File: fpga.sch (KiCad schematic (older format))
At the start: 18 parts, among them U5 ICE40UP5K-SG48ITR, U6 LY68L6400

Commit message: Change pinout of expansion header close to board edge to be fully ground instead of gnd + 3.3v (& update component references)
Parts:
- C15, C16, C17, C18, C19, C20, C21, C22: symbol Device:C_Small -> mch2021-rescue:C_Small-Device
- R31, R32, R33, R34, R35, R36: symbol Device:R_Small -> mch2021-rescue:R_Small-Device
- RN4, RN5: symbol Device:R_Pack04 -> mch2021-rescue:R_Pack04-Device
- U5: symbol FPGA_Lattice:ICE40UP5K-SG48ITR -> mch2021-rescue:ICE40UP5K-SG48ITR-FPGA_Lattice
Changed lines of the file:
@@
 $EndDescr
 $Comp
-L FPGA_Lattice:ICE40UP5K-SG48ITR U5
+L mch2021-rescue:ICE40UP5K-SG48ITR-FPGA_Lattice U5
 U 1 1 5F52B856
 P 1850 6100
@@
 $EndComp
 $Comp
-L FPGA_Lattice:ICE40UP5K-SG48ITR U5
+L mch2021-rescue:ICE40UP5K-SG48ITR-FPGA_Lattice U5
 U 2 1 5F52DB74
 P 3500 6100
@@
 $EndComp
 $Comp
-L FPGA_Lattice:ICE40UP5K-SG48ITR U5
+L mch2021-rescue:ICE40UP5K-SG48ITR-FPGA_Lattice U5
 U 3 1 5F52F020
 P 9000 3900
@@
 $EndComp
 $Comp
-L FPGA_Lattice:ICE40UP5K-SG48ITR U5
+L mch2021-rescue:ICE40UP5K-SG48ITR-FPGA_Lattice U5
 U 4 1 5F5301DA
 P 2650 1200
@@
 $EndComp
 $Comp
-L Device:R_Small R33
+L mch2021-rescue:R_Small-Device R33
 U 1 1 5F537E5C
 P 1700 1350
@@
 $EndComp
 $Comp
-L Device:C_Small C16
+L mch2021-rescue:C_Small-Device C16
 U 1 1 5F54E79A
 P 1300 1700
@@
 $EndComp
 $Comp
-L Device:C_Small C17
+L mch2021-rescue:C_Small-Device C17
 U 1 1 5F54FA10
 P 1700 1700
@@
 $EndComp
 $Comp
-L Device:C_Small C18
+L mch2021-rescue:C_Small-Device C18
 U 1 1 5F551B90
 P 2100 1700
@@
 $EndComp
 $Comp
-L power:GND #PWR084
+L mch2021-rescue:GND-power #PWR084
 U 1 1 5F553535
 P 2100 1800
@@
 $EndComp
 $Comp
-L power:GND #PWR080
+L mch2021-rescue:GND-power #PWR080
 U 1 1 5F553952
 P 1700 1800
@@
 $EndComp
 $Comp
-L power:GND #PWR078
+L mch2021-rescue:GND-power #PWR078
 U 1 1 5F553E39
 P 1300 1800
@@
 Connection ~ 1300 1200
 $Comp
-L power:+1V2 #PWR075
+L mch2021-rescue:+1V2-power #PWR075
 U 1 1 5F564804
 P 900 1000
@@
 $EndComp
 $Comp
-L power:GND #PWR088
+L mch2021-rescue:GND-power #PWR088
 U 1 1 5F565850
 P 3150 1800
@@
 	3150 1200 3050 1200
 $Comp
-L power:+3.3V #PWR091
+L mch2021-rescue:+3.3V-power #PWR091
 U 1 1 5F57B8C0
 P 3500 5000
@@
 FPGA_CDONE
 $Comp
-L power:GND #PWR077
+L mch2021-rescue:GND-power #PWR077
 U 1 1 5F58383F
 P 1100 3150
@@
 $EndComp
 $Comp
-L Device:R_Small R31
+L mch2021-rescue:R_Small-Device R31
 U 1 1 5F59314F
 P 1100 3050
@@
 FPGA_RESET
 $Comp
-L Device:R_Small R32
+L mch2021-rescue:R_Small-Device R32
 U 1 1 5F5BBEB5
 P 1400 2700
@@
 FPGA_CDONE
 $Comp
-L power:+3.3V #PWR079
+L mch2021-rescue:+3.3V-power #PWR079
 U 1 1 5F5BD259
 P 1400 2600
@@
 LCD_FMARK
 $Comp
-L power:+3.3V #PWR082
+L mch2021-rescue:+3.3V-power #PWR082
 U 1 1 60CF7467
 P 1850 5000
@@
 RGB0
 $Comp
-L power:+3.3V #PWR094
+L mch2021-rescue:+3.3V-power #PWR094
 U 1 1 5F32B7AB
 P 9000 3200
@@
 	10500 1750 10500 1800
 $Comp
-L power:GND #PWR099
+L mch2021-rescue:GND-power #PWR099
 U 1 1 5F3AAB21
 P 10500 1800
@@
 $EndComp
 $Comp
-L Device:R_Small R36
+L mch2021-rescue:R_Small-Device R36
 U 1 1 5F436AA9
 P 9450 1050
@@
 	9450 1250 9450 1150
 $Comp
-L power:+3.3V #PWR095
+L mch2021-rescue:+3.3V-power #PWR095
 U 1 1 5F439DDC
 P 9450 950
@@
 $EndComp
 $Comp
-L power:+3.3V #PWR098
+L mch2021-rescue:+3.3V-power #PWR098
 U 1 1 5F43A076
 P 10500 950
@@
 	9550 1750 9350 1750
 $Comp
-L Device:C_Small C21
+L mch2021-rescue:C_Small-Device C21
 U 1 1 5F472EE7
 P 4700 5100
@@
 $EndComp
 $Comp
-L power:GND #PWR093
+L mch2021-rescue:GND-power #PWR093
 U 1 1 5F473D9D
 P 4700 5200
@@
 $EndComp
 $Comp
-L power:+3.3V #PWR092
+L mch2021-rescue:+3.3V-power #PWR092
 U 1 1 5F473F7E
 P 4700 5000
@@
 $EndComp
 $Comp
-L Device:C_Small C22
+L mch2021-rescue:C_Small-Device C22
 U 1 1 5F47D064
 P 9550 3300
@@
 $EndComp
 $Comp
-L power:GND #PWR097
+L mch2021-rescue:GND-power #PWR097
 U 1 1 5F47D06A
 P 9550 3400
@@
 $EndComp
 $Comp
-L power:+3.3V #PWR096
+L mch2021-rescue:+3.3V-power #PWR096
 U 1 1 5F47D070
 P 9550 3200
@@
 $EndComp
 $Comp
-L Device:C_Small C20
+L mch2021-rescue:C_Small-Device C20
 U 1 1 5F47E26A
 P 3450 1700
@@
 $EndComp
 $Comp
-L power:GND #PWR090
+L mch2021-rescue:GND-power #PWR090
 U 1 1 5F47E270
 P 3450 1800
@@
 $EndComp
 $Comp
-L power:+3.3V #PWR089
+L mch2021-rescue:+3.3V-power #PWR089
 U 1 1 5F47E276
 P 3450 1600
@@
 $EndComp
 $Comp
-L Device:C_Small C19
+L mch2021-rescue:C_Small-Device C19
 U 1 1 5F489EE6
 P 2300 5100
@@
 $EndComp
 $Comp
-L power:GND #PWR087
+L mch2021-rescue:GND-power #PWR087
 U 1 1 5F489EEC
 P 2300 5200
@@
 $EndComp
 $Comp
-L power:+3.3V #PWR086
+L mch2021-rescue:+3.3V-power #PWR086
 U 1 1 5F489EF2
 P 2300 5000
@@
 $EndComp
 $Comp
-L Device:C_Small C15
+L mch2021-rescue:C_Small-Device C15
 U 1 1 5F48A8F4
 P 900 1700
@@
 $EndComp
 $Comp
-L power:GND #PWR076
+L mch2021-rescue:GND-power #PWR076
 U 1 1 5F48A8FA
 P 900 1800
@@
 PMOD_7
 $Comp
-L Device:R_Pack04 RN5
+L mch2021-rescue:R_Pack04-Device RN5
 U 1 1 5FD85945
 P 7300 4300
@@
 IRQ
 $Comp
-L Device:R_Small R34
+L mch2021-rescue:R_Small-Device R34
 U 1 1 5F54C08B
 P 1750 2700
@@
 $EndComp
 $Comp
-L power:+3.3V #PWR081
+L mch2021-rescue:+3.3V-power #PWR081
 U 1 1 5F54C091
 P 1750 2600
@@
 RGB1
 $Comp
-L Device:R_Small R35
+L mch2021-rescue:R_Small-Device R35
 U 1 1 5F503F4E
 P 2050 2700
@@
 SPI_CS
 $Comp
-L power:+3.3V #PWR083
+L mch2021-rescue:+3.3V-power #PWR083
 U 1 1 5F89A681
 P 2050 2600
@@
 $EndComp
 $Comp
-L power:+3.3V #PWR085
+L mch2021-rescue:+3.3V-power #PWR085
 U 1 1 5F8E28AC
 P 2250 1100
@@
 I2S_LR
 $Comp
-L Device:R_Pack04 RN4
+L mch2021-rescue:R_Pack04-Device RN4
 U 1 1 5FD84D43
 P 7300 3900

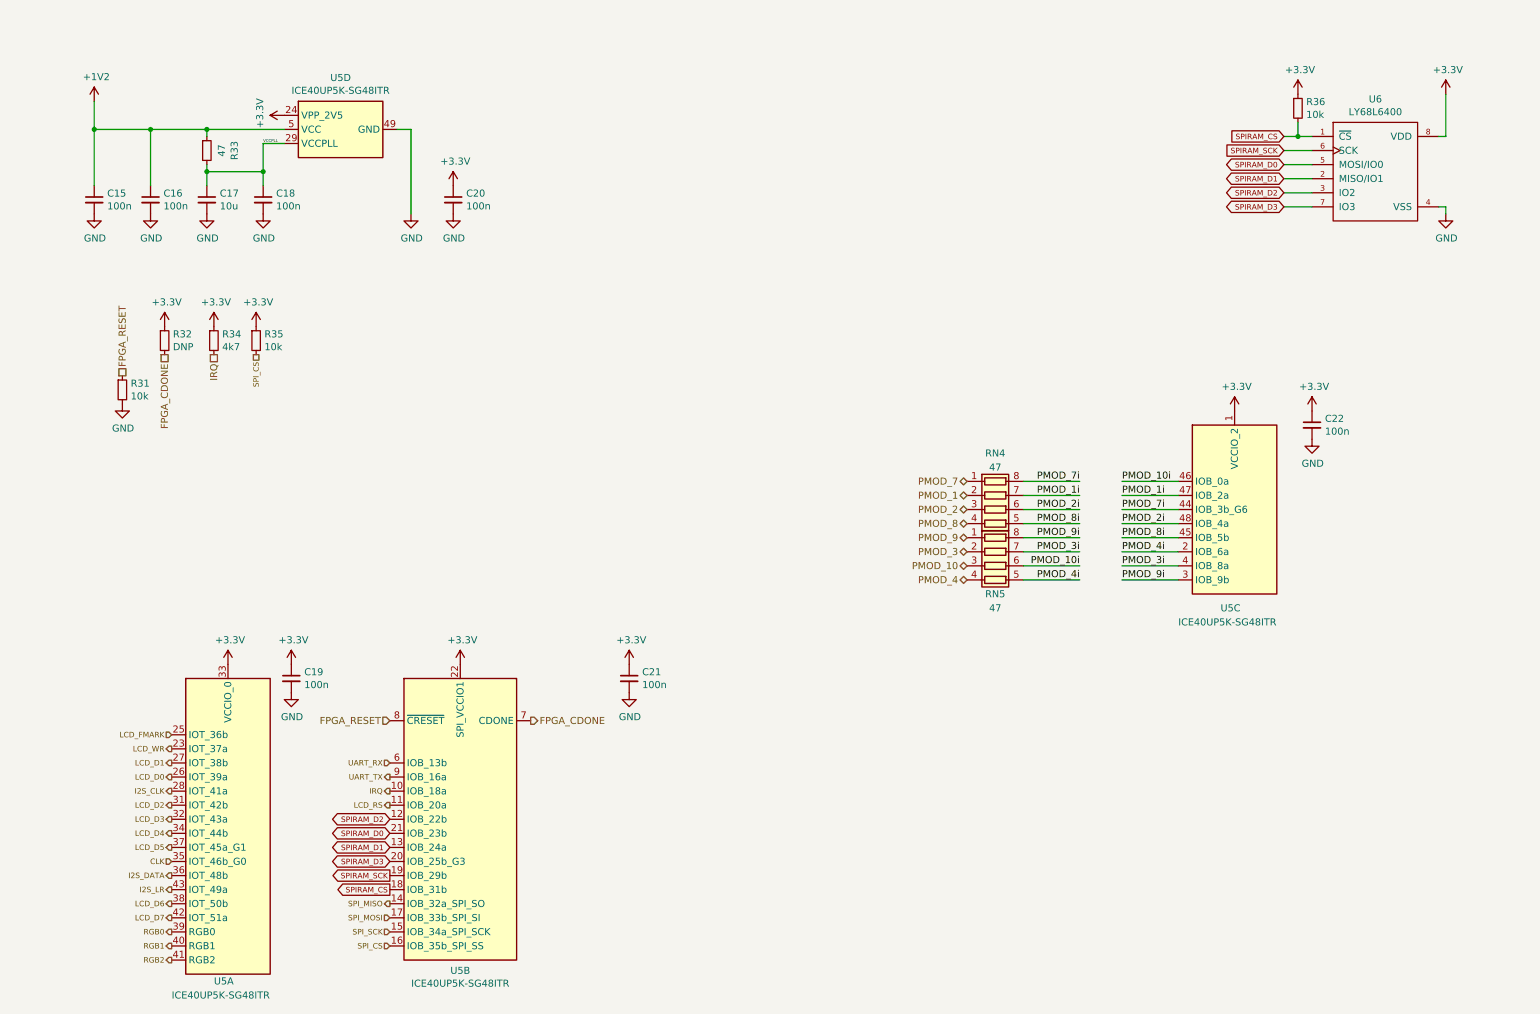
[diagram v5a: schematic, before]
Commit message: Add flash chip footprint, fix routing of flash chip, fix DRC errors
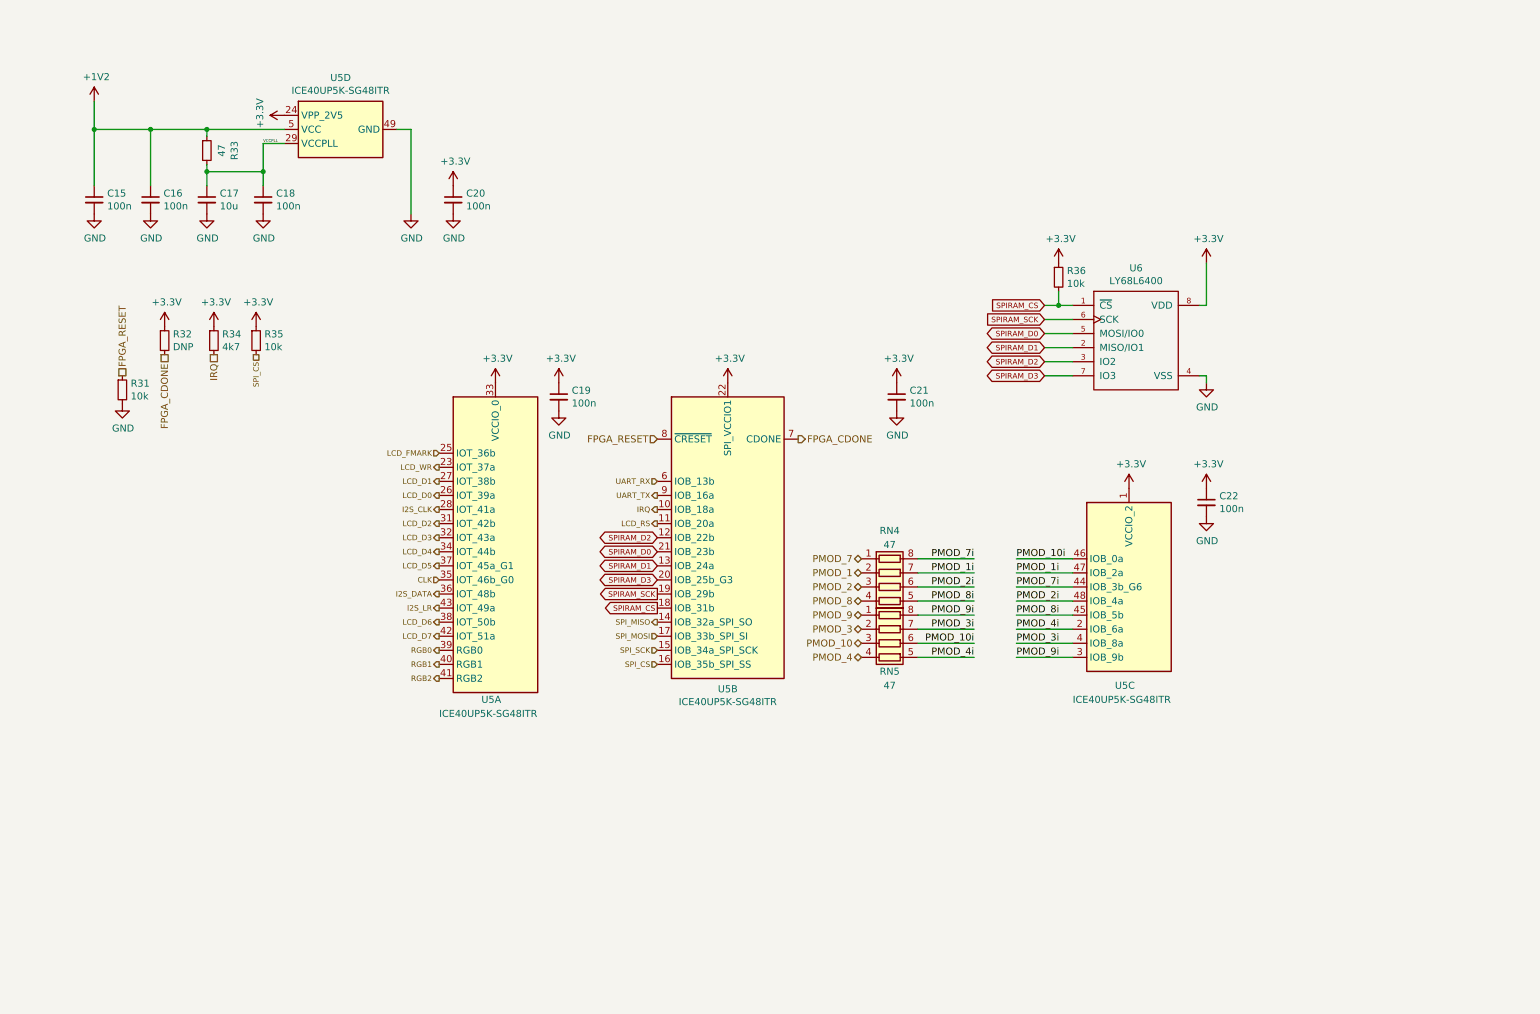
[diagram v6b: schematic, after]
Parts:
- U6: footprint Package_SO:SOIC-8-1EP_3.9x4.9mm_P1.27mm_EP2.41x3.81mm -> Package_SO:SOIC-8_3.9x4.9mm_P1.27mm
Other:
- moved on the sheet: C19, C21, C22, R36, RN4, RN5, U5A, U5B, U5C, U6

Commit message: Add oscillator for ICE40, add testpoints for unused RP2040 pins
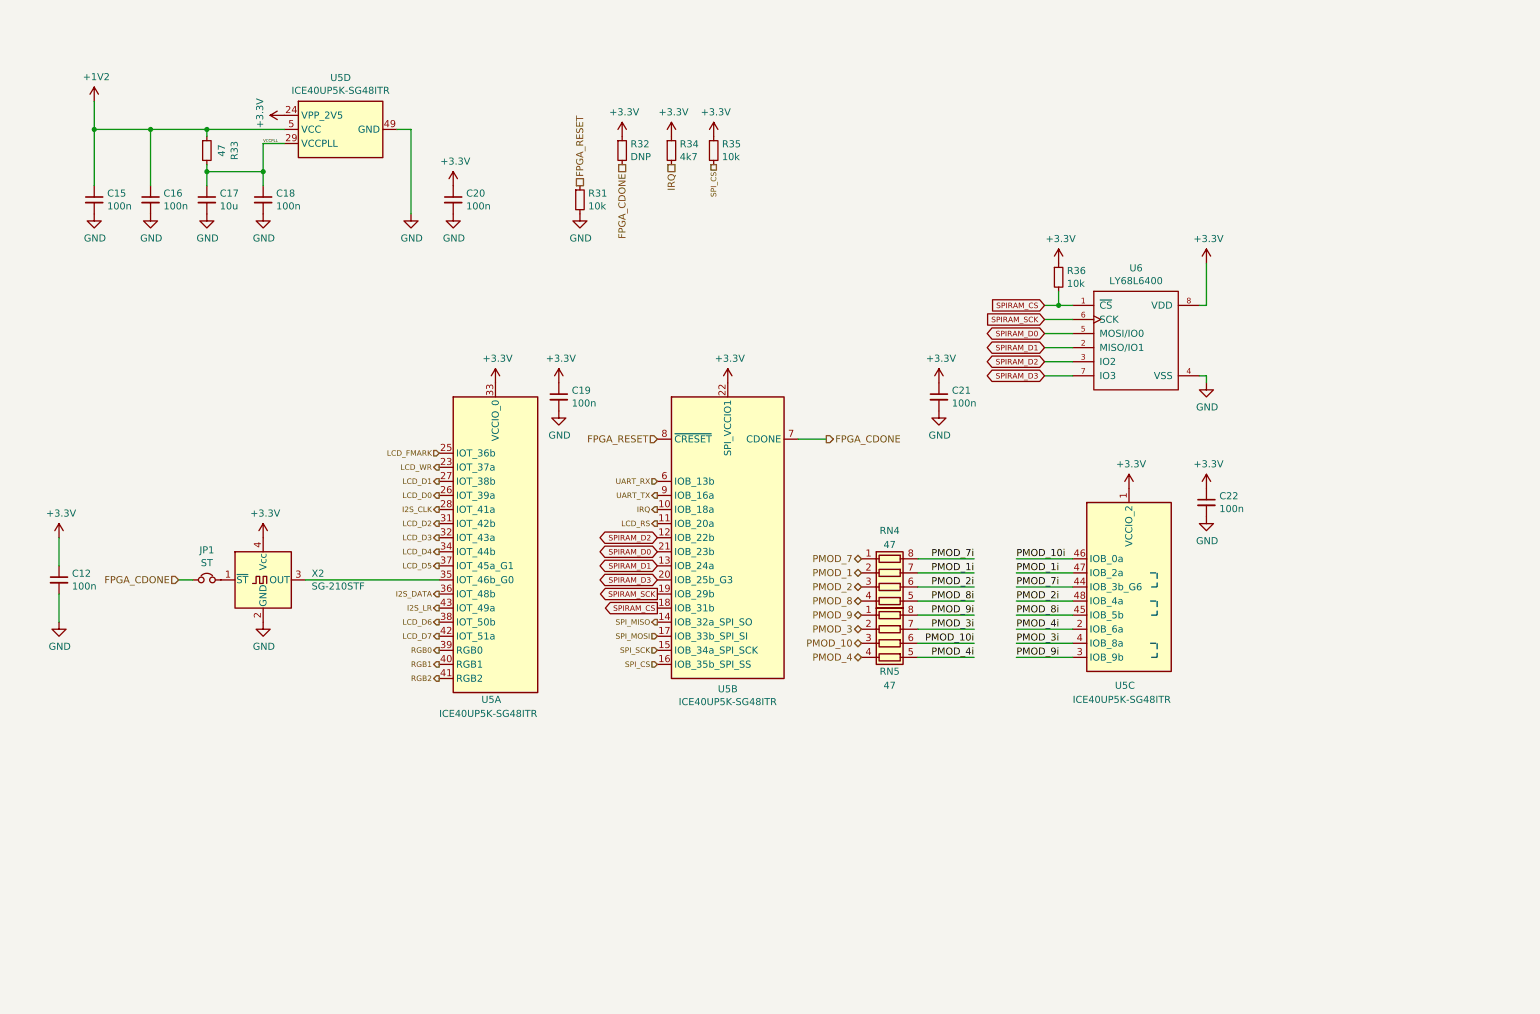
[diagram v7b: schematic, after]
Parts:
- added C12: 100n, Capacitor_SMD:C_0402_1005Metric, symbol mch2021-rescue:C_Small-Device
- added JP1: ST, Jumpers:SMT-JUMPER_2_NC_PASTE_NO-SILK, symbol Device:Jumper_NC_Small
- added X2: SG-210STF, Oscillator:Oscillator_SMD_SeikoEpson_SG210-4Pin_2.5x2.0mm, symbol Oscillator:SG-210STF
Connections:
- net +3V3: now also C12.1, X2.4 (Vcc)
- net FPGA_CDONE: now also JP1.1
- net GND: now also C12.2, X2.2 (GND)
- net CLK: no longer names the net of U5.35 (IOT_46b_G0)
- net CLK: now also X2.3 (OUT)
- new net: JP1.2, X2.1 (~ST~)
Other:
- moved on the sheet: C21, R31, R32, R34, R35
